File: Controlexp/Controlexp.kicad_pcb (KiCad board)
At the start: 2 copper layers, 100.3 x 100.3 mm, 26 parts, among them J1 SMA_CONNECTOR, J4 530470510, J5 Power Connector, J6 Pressure sensor, J7 POWER PROBE, U2 RFM95W, U3 TPS62162DSG, U4 BME680, U5 XIAO-nRF52840-DIP

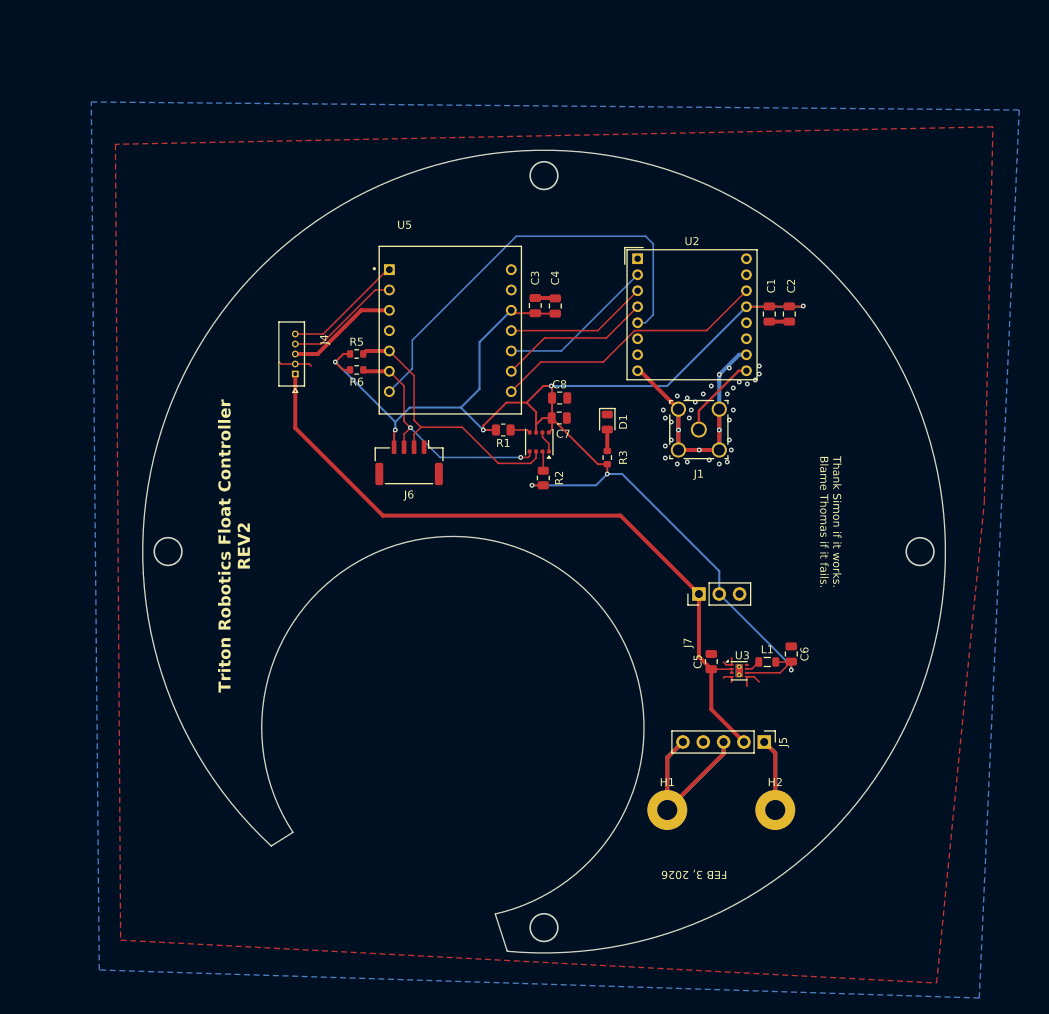
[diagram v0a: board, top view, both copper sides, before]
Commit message: fresh board
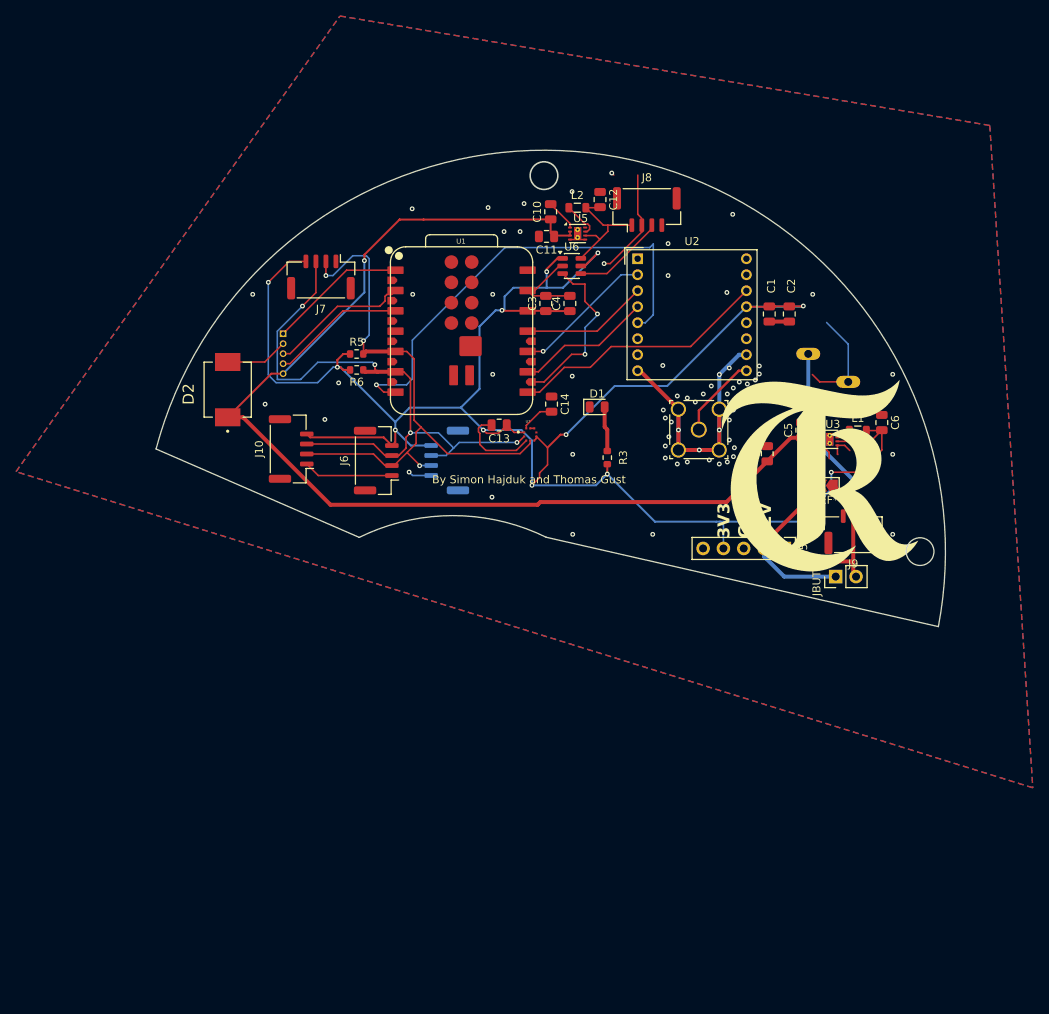
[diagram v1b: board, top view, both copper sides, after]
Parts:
- removed C7: 0.1uF, Capacitor_SMD:C_0805_2012Metric
- removed C8: 10uF, Capacitor_SMD:C_0805_2012Metric
- removed H1: GND, MountingHole:MountingHole_2.5mm_Pad
- removed H2: 12V, MountingHole:MountingHole_2.5mm_Pad
- removed R1, R2: 10k, Resistor_SMD:R_0805_2012Metric
- removed U4: BME680, Package_LGA:Bosch_LGA-8_3x3mm_P0.8mm_ClockwisePinNumbering
- added C10: 220 uF, Capacitor_SMD:C_0805_2012Metric, F.Cu at (141.9, 47.2)
- added C11: 10uF, 25V, Capacitor_SMD:C_0805_2012Metric, F.Cu at (141.4, 50.3)
- added C12: 22uF, 10V, Capacitor_SMD:C_0805_2012Metric, F.Cu at (148.1, 45.7)
- added C13: 100nF, Capacitor_SMD:C_0805_2012Metric, F.Cu at (135.5, 73.9)
- added C14: 100nF, Capacitor_SMD:C_0805_2012Metric, F.Cu at (142.0, 71.3)
- added C9: 220 uF, Capacitor_SMD:C_0805_2012Metric, F.Cu at (169.0, 77.5)
- added D2: SS34, SS34:DIOM7959X265N, F.Cu at (101.5, 69.5)
- added J10: Extra sensor TOP, Connector_JST:JST_GH_BM04B-GHS-TBT_1x04-1MP_P1.25mm_Vertical, F.Cu at (109.5, 76.9)
- added J11: Extra sensor BOTTOM, Connector_JST:JST_GH_BM04B-GHS-TBT_1x04-1MP_P1.25mm_Vertical, B.Cu at (128.9, 78.3)
- added J2: Conn_01x02, 250-202:P-250-202, B.Cu at (175.4, 67.5)
- added J8: LED, Connector_JST:JST_GH_BM04B-GHS-TBT_1x04-1MP_P1.25mm_Vertical, F.Cu at (153.9, 46.9)
- added J9: PWRCONN, Connector_JST:JST_GH_BM03B-GHS-TBT_1x03-1MP_P1.25mm_Vertical, F.Cu at (179.7, 87.2)
- added JBUTT1: Conn_01x02, Connector_PinHeader_2.54mm:PinHeader_1x02_P2.54mm_Vertical, F.Cu at (177.6, 92.8)
- added L2: 2.2uH, Inductor_SMD:L_0805_2012Metric, F.Cu at (145.3, 46.7)
- added REF**: SolderJumper-2_P1.3mm_Open_TrianglePad1.0x1.5mm, Jumper:SolderJumper-2_P1.3mm_Open_TrianglePad1.0x1.5mm, F.Cu at (176.6, 81.5)
- added U1: XIAO-ESP32-S3-Plus-SMD, New_XIAO_Series_Footprints:XIAO-ESP32-S3-Plus-SMD, F.Cu at (130.8, 62.1)
- added U6: SN74LVC1T45DBV, Package_TO_SOT_SMD:SOT-23-6, F.Cu at (144.6, 54.0)
- added U7: BMP388, BMP388:XDCR_BMP388, F.Cu at (139.4, 75.1)
- J1: value SMA_CONNECTOR -> Conn_Coaxial_Small; footprint SMASMA2:CONN_RF2-04A-T-00-50-G_ADM -> SMAv2:CONN_RF2-04A-T-00-50-G_ADM
- J4: moved to B.Cu
- J7: value POWER PROBE -> ToF sensor; footprint Connector_PinHeader_2.54mm:PinHeader_1x03_P2.54mm_Vertical -> Connector_JST:JST_GH_BM04B-GHS-TBT_1x04-1MP_P1.25mm_Vertical
- U5: value XIAO-nRF52840-DIP -> TPS62163DSG; footprint MCU_SEED:MODULE_113991054 -> Package_SON:WSON-8-1EP_2x2mm_P0.5mm_EP0.9x1.6mm_ThermalVias
- moved J7 61.7 mm to (113.2, 55.4), turned to 180 degrees
- moved C5 31.1 mm to (173.3, 74.5)
- moved C6 31.1 mm to (183.3, 73.6)
- moved L1 31.1 mm to (180.3, 74.6)
- moved U3 31.1 mm to (176.8, 75.7)
- moved J5 24.3 mm to (171.1, 89.3)
- moved U5 20.0 mm to (145.3, 49.9)
- moved J4 5.26 mm to (108.5, 62.5), turned to 90 degrees
- moved J6 4.11 mm to (120.1, 78.3), turned to 90 degrees
- moved D1 2.27 mm to (147.7, 71.6), turned to 0 degrees
- moved C4 1.85 mm to (144.3, 58.7)
- moved C3 1.34 mm to (141.3, 58.7)
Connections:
- J4 pad 1: +12V -> /PWM
- J4 pad 3: /PWM -> /DIR
- J4 pad 4: /DIR -> /FEEDBACK
- J4 pad 5: /FEEDBACK -> +12V
- J5 pad 1: /MAIN -> +12V
- J5 pad 4: +3V3 -> +3.3V
- J6 pad 2: /SDA -> /BMPSDA
- J6 pad 3: /SCL -> /BMPSCL
- J7 pad 1: +12V -> GND
- J7 pad 2: +3.3V -> /BMPSDA
- J7 pad 3: GND -> /BMPSCL
- R5 pad 1: /SDA -> /BMPSDA
- R6 pad 1: /SCL -> /BMPSCL
- U5 pad 1: /FEEDBACK -> GND
- U5 pad 2: /DIR -> +12V
- U5 pad 3: /PWM -> +12V
- U5 pad 4: /PWR_SWITCH -> GND
- U5 pad 5: /SDA -> GND
- U5 pad 6: /SCL -> +5V
- U5 pad 7: /NSS -> Net-(U5-SW)
- U5 pad 8: /INT -> unconnected-(U5-PG-Pad8)
- U5 pad 9: /SCK -> GND
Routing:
- net +12V: track 89.7 -> 215.2 mm, vias 0 -> 2
- net /BMPSCL: track 0.00 -> 80.1 mm, vias 0 -> 4
- net +3.3V: track 186.7 -> 261.9 mm, vias 8 -> 12
- net /BMPSDA: track 0.00 -> 73.8 mm, vias 0 -> 3
- net /SDA: track 34.8 -> 0.00 mm
- net /SCL: track 31.3 -> 0.00 mm, vias 2 -> 0
- net GND: track 106.7 -> 133.9 mm, vias 34 -> 64
- net /LEDSERIAL: track 0.00 -> 21.6 mm, vias 0 -> 2
- net /MAIN: track 18.1 -> 0.00 mm
- net +5V: track 0.00 -> 15.9 mm
- net /DIN: track 0.00 -> 11.6 mm
- net Net-(U5-SW): track 0.00 -> 4.63 mm
- net Net-(U7-VDD): track 0.00 -> 4.23 mm
- net /NSS: track 54.7 -> 58.7 mm, vias 0 -> 1
- net /PWM: track 14.0 -> 17.3 mm
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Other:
- board size 100.3 x 100.3 mm -> 98.7 x 59.5 mm
- board text added: "12V"
- board text added: "3V3"
- board text added: "By Simon Hajduk and Thomas Gust"
- board text added: "GND"
- board text removed: "FEB 3, 2026"
- board text removed: "Thank Simon if it works. Blame Thomas if it fails."
- board text removed: "Triton Robotics Float Controller REV2"
